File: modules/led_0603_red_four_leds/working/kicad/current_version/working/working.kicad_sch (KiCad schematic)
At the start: 8 parts

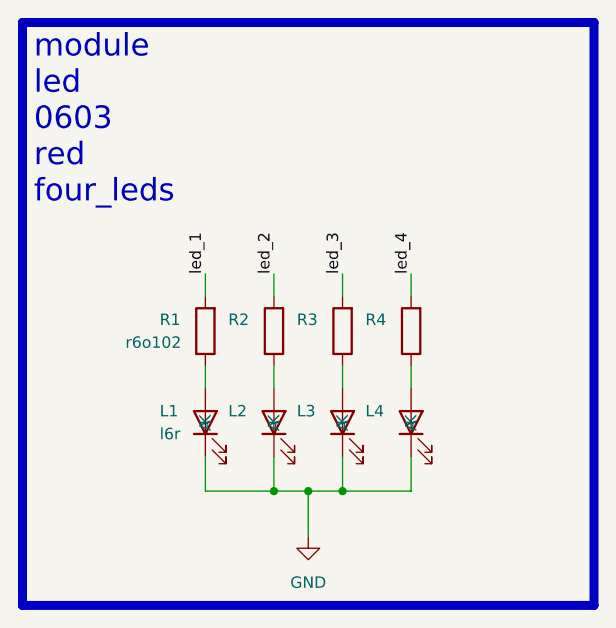
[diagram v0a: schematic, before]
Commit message: gitignore update mainly and update
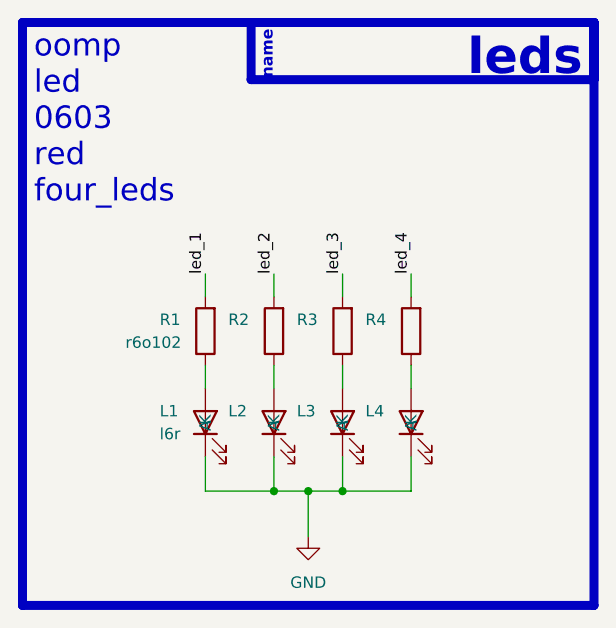
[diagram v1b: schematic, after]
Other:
- note added: "leds"
- note added: "name"
- note added: "oomp led 0603 red four_leds"
- note removed: "module led 0603 red four_leds"
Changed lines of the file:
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@@
     (stroke (width 0) (type default))
+  )
+  (rectangle (start 144.78 58.42) (end 182.88 64.77)
+    (stroke (width 1) (type default))
+    (fill (type color) (color 0 0 0 0))
   )
   (rectangle (start 119.38 58.42) (end 182.88 123.19)
@@
     (fill (type none))
   )
-  (text "module\nled\n0603\nred\nfour_leds\n" (at 120.65 78.74 0)
+  (text "name" (at 147.32 64.77 90)
+    (effects (font (size 1.27 1.27) (thickness 0.254) bold (color 255 255 255 1)) (justify left bottom))
+  )
+  (text "oomp\nled\n0603\nred\nfour_leds\n" (at 120.65 78.74 0)
     (effects (font (size 2.5 2.5)) (justify left bottom))
   )
+  (text "leds" (at 181.61 64.77 0)
+    (effects (font (size 4 4) (thickness 0.8) bold (color 255 255 255 1)) (justify right bottom))
+  )
   (label "led_2" (at 147.32 86.36 90) (fields_autoplaced)
